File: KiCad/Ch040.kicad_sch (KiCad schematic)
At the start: 17 parts, among them J1 Conn_01x09, J2 Conn_01x09, J3 Conn_01x10, J4 Conn_01x02

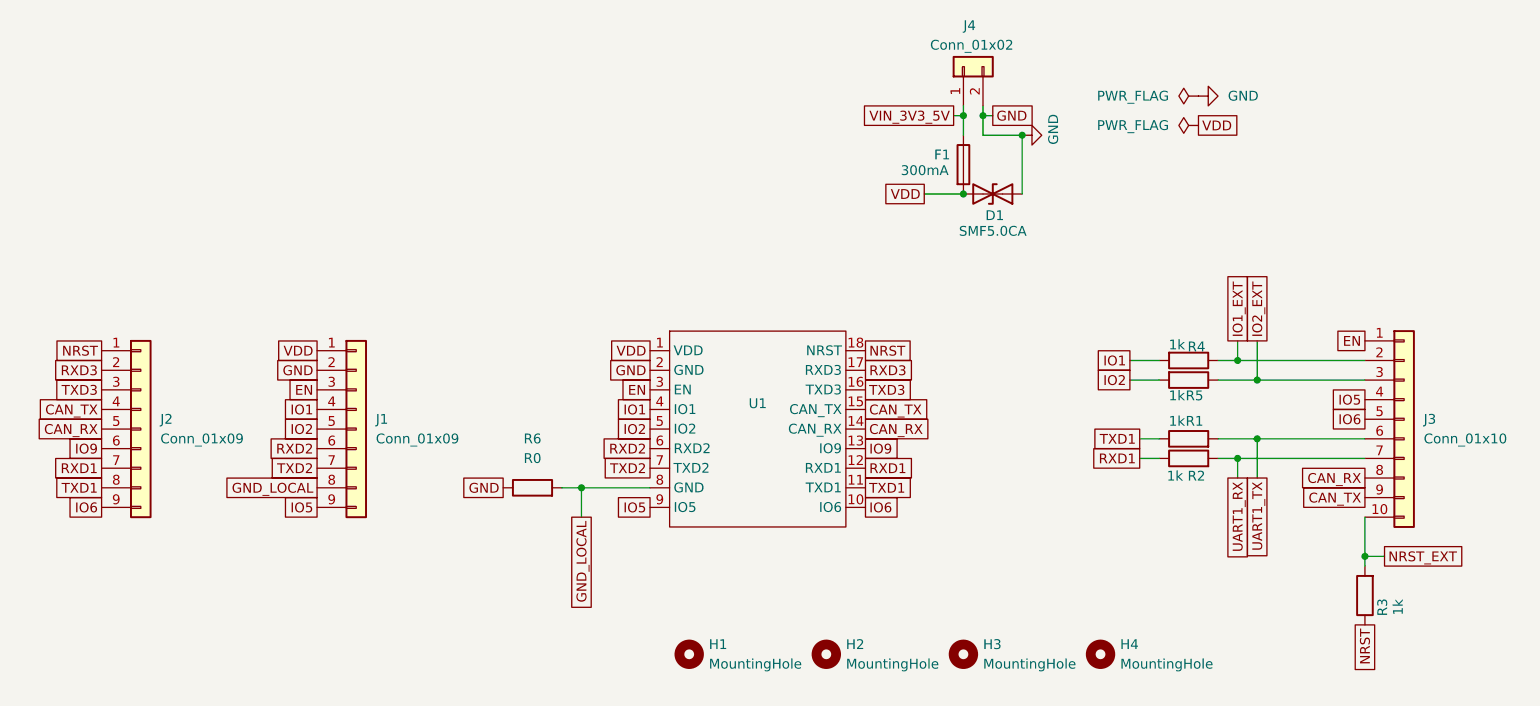
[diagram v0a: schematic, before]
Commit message: Add files via upload
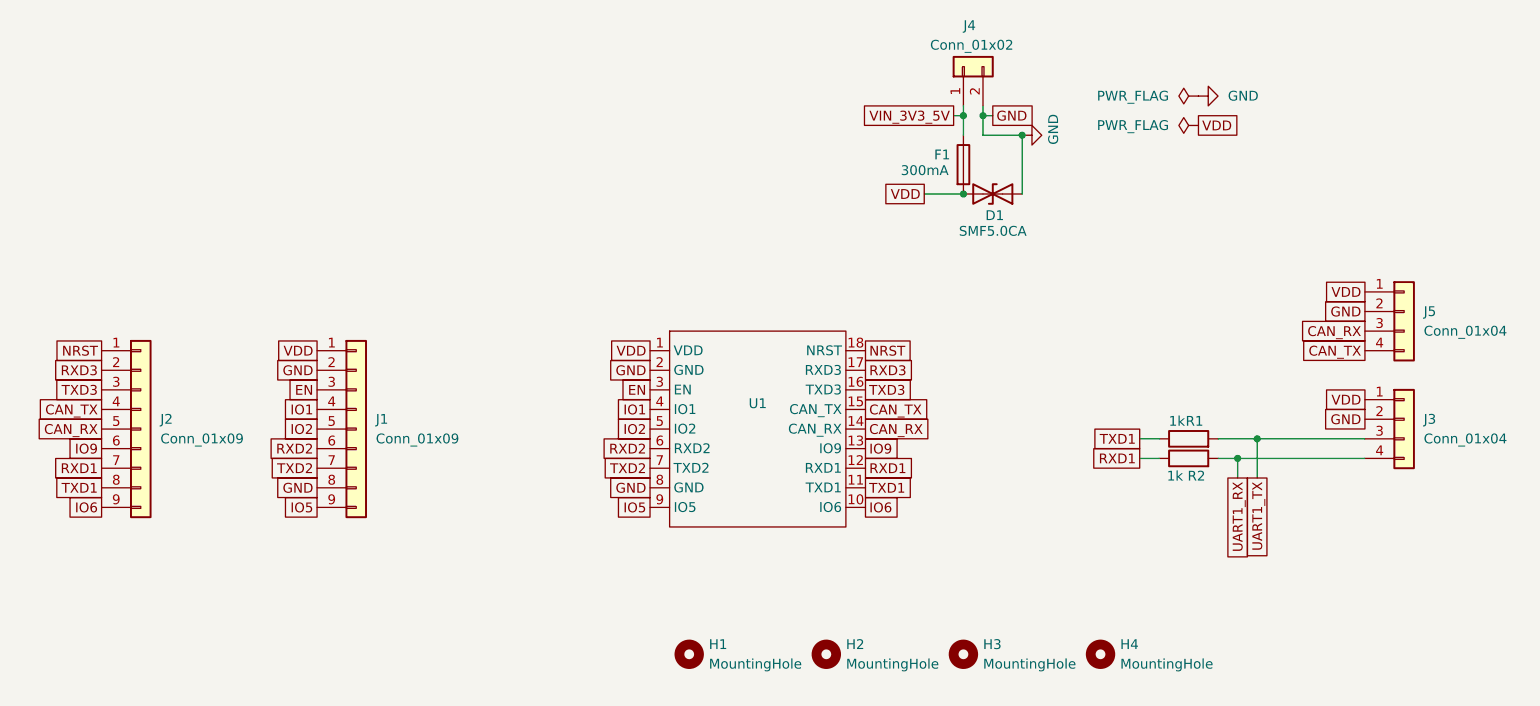
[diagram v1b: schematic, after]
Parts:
- removed J3: Conn_01x10, Connector_JST:JST_GH_SM10B-GHS-TB_1x10-1MP_P1.25mm_Horizontal, symbol Connector_Generic:Conn_01x10
- removed R3, R4, R5: 1k, Resistor_SMD:R_0805_2012Metric, symbol Device:R
- removed R6: R0, Resistor_THT:R_Axial_DIN0207_L6.3mm_D2.5mm_P10.16mm_Horizontal, symbol Device:R
- added J3, J5: Conn_01x04, Connector_JST:JST_GH_SM04B-GHS-TB_1x04-1MP_P1.25mm_Horizontal, symbol Connector_Generic:Conn_01x04
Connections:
- net GND_LOCAL is gone; now on net GND: J1.8 (Pin_8), U1.8 (GND)
- net CAN_RX: now also J5.3 (Pin_3)
- net CAN_TX: now also J5.4 (Pin_4)
- net GND: now also J3.2 (Pin_2), J5.2 (Pin_2)
- net UART1_RX: now also J3.4 (Pin_4)
- net UART1_TX: now also J3.3 (Pin_3)
- net VDD: now also J3.1 (Pin_1), J5.1 (Pin_1)
